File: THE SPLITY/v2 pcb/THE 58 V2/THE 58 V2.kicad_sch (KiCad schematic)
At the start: 146 parts, among them J1 Conn_01x02_Socket, J2 Conn_01x02_Socket, SW1 Switch, SW2 Switch, SW3 Switch, SW4 Switch, U1 Nice_Nano_V2, U2 Nice_Nano_V2, U3 TRRS, U4 TRRS

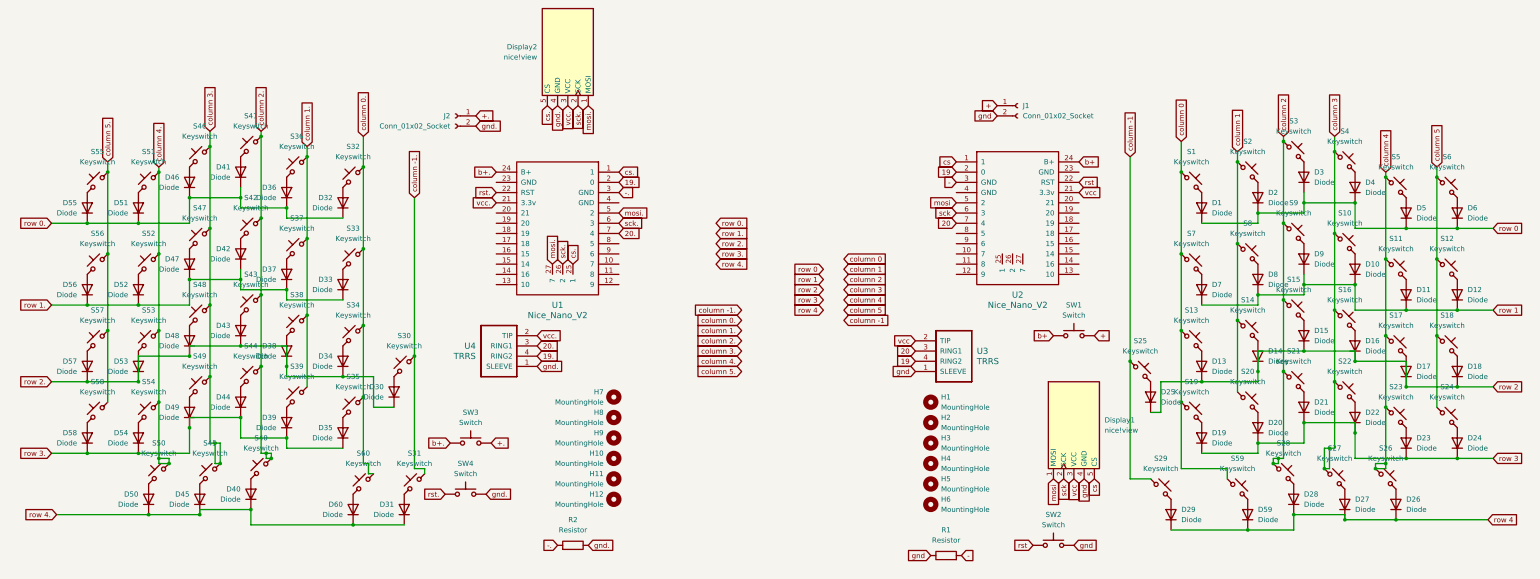
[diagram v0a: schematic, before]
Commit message: almost finished the pcb
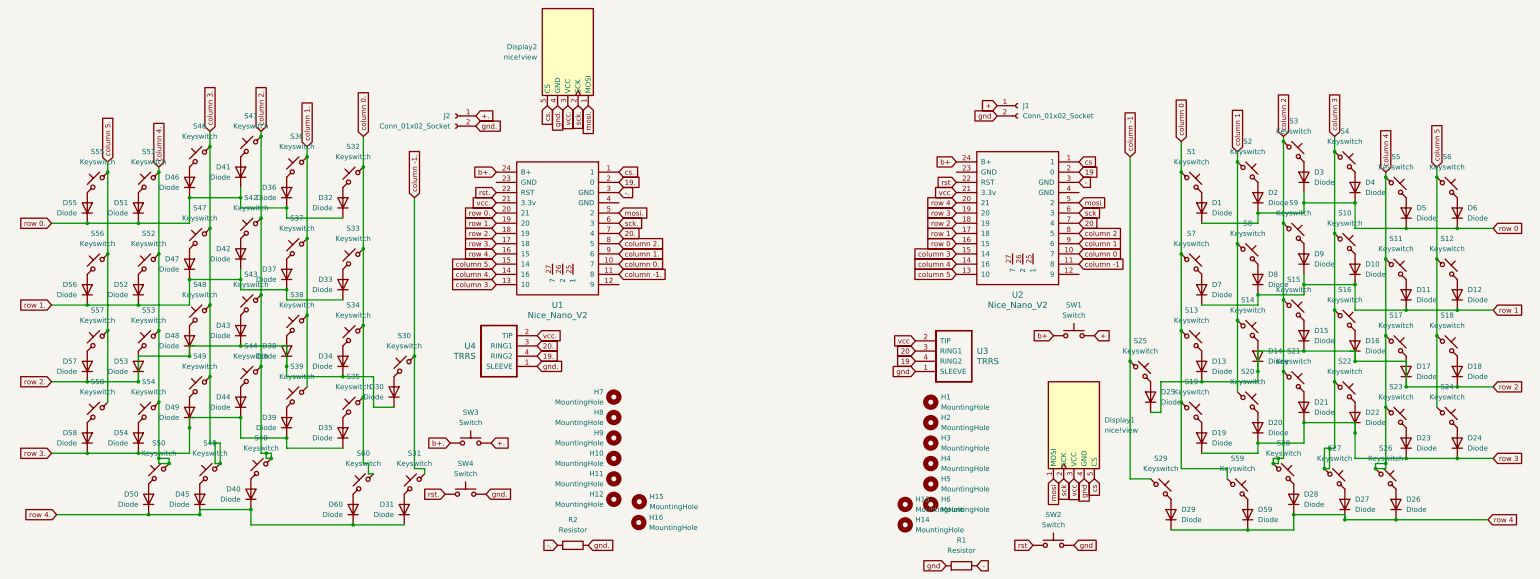
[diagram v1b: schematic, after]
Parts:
- added H13, H14, H15, H16: MountingHole, MountingHole:MountingHole_2.2mm_M2, symbol Mechanical:MountingHole
- R1, R2: footprint (none) -> Resistor_THT:R_Axial_DIN0207_L6.3mm_D2.5mm_P7.62mm_Horizontal
- S60: footprint ScottoKeebs_MX:MX_PCB_1.00u_Reversable -> ScottoKeebs_MX:MX_PCB_1.00u
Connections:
- net -: now also R1.1; no longer R1.2
- net column -1: now also U2.11 (8)
- net column -1.: now also U1.11 (8)
- net column 0: now also U2.10 (7)
- net column 0.: now also U1.10 (7)
- net column 1: now also U2.9 (6)
- net column 1.: now also U1.9 (6)
- net column 2: now also U2.8 (5)
- net column 2.: now also U1.8 (5)
- net column 3: now also U2.15 (14)
- net column 3.: now also U1.13 (10)
- net column 4: now also U2.14 (16)
- net column 4.: now also U1.14 (16)
- net column 5: now also U2.13 (10)
- net column 5.: now also U1.15 (14)
- net cs.: no longer U1.25 (1)
- net gnd: now also R1.2; no longer R1.1
- net mosi.: no longer U1.27 (7)
- net row 0: now also U2.16 (15)
- net row 0.: now also U1.20 (21)
- net row 1: now also U2.17 (18)
- net row 1.: now also U1.19 (20)
- net row 2: now also U2.18 (19)
- net row 2.: now also U1.18 (19)
- net row 3: now also U2.19 (20)
- net row 3.: now also U1.17 (18)
- net row 4: now also U2.20 (21)
- net row 4.: now also U1.16 (15)
- net sck.: no longer U1.26 (2)
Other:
- moved on the sheet: R1
